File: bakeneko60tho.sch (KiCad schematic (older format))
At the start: 14 parts

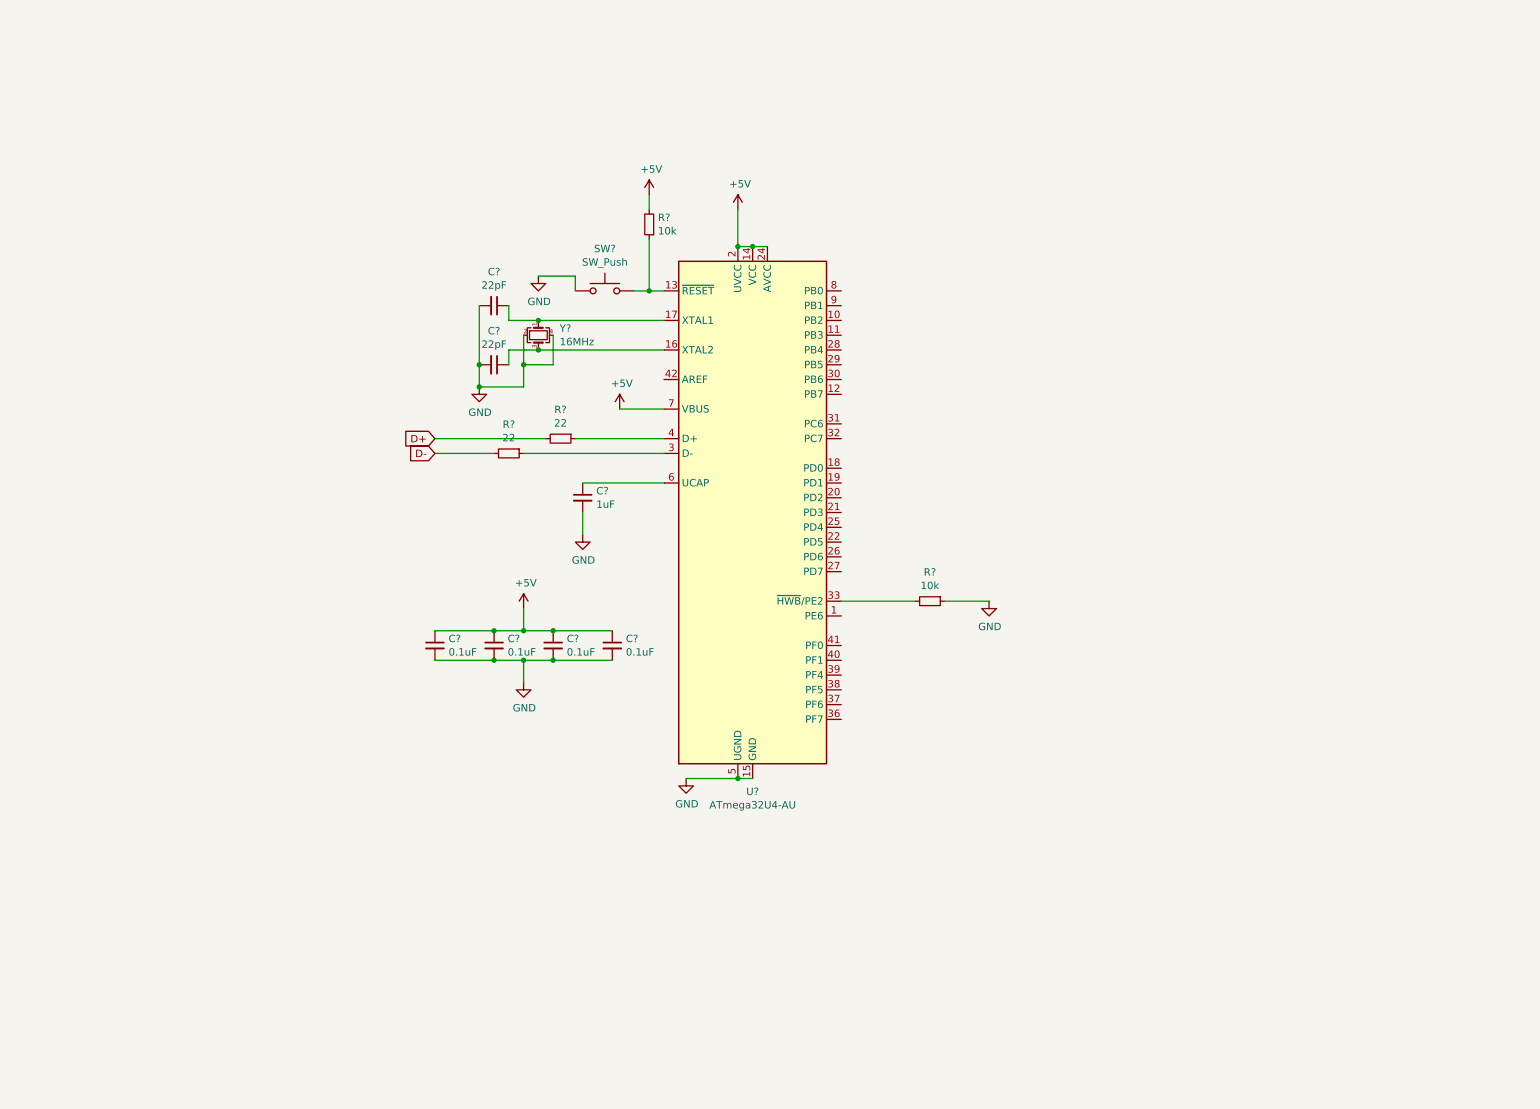
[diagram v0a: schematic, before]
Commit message: assign footprints
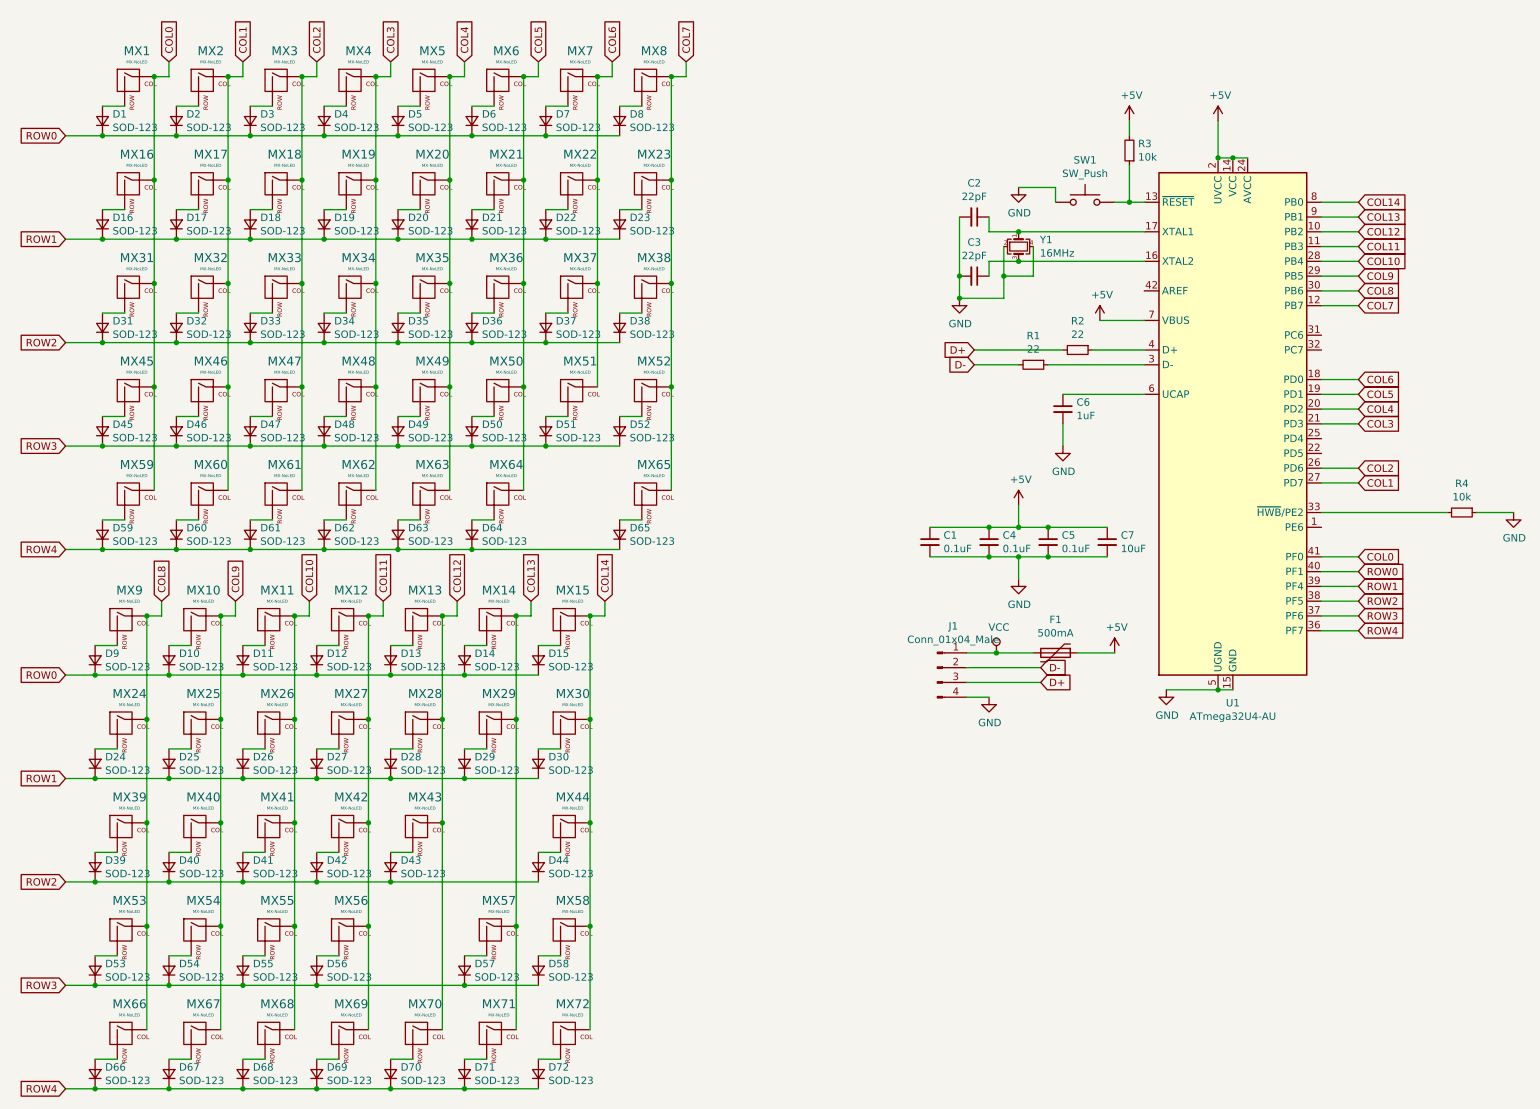
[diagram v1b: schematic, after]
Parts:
- added D1, D10, D11, D12, D13, D14, D15, D16, D17, D18, D19, D2, D20, D21, D22, D23, D24, D25, D26, D27, D28, D29, D3, D30, D31, D32, D33, D34, D35, D36, D37, D38, D39, D4, D40, D41, D42, D43, D44, D45, D46, D47, D48, D49, D5, D50, D51, D52, D53, D54, D55, D56, D57, D58, D59, D6, D60, D61, D62, D63, D64, D65, D66, D67, D68, D69, D7, D70, D71, D72, D8, D9: SOD-123, Diode_SMD:D_SOD-123, symbol Device:D_Small
- added F1: 500mA, Fuse:Fuse_1206_3216Metric, symbol Device:Polyfuse
- added J1: Conn_01x04_Male, Connector_PinHeader_1.00mm:PinHeader_1x04_P1.00mm_Horizontal, symbol Connector:Conn_01x04_Male
- added MX1, MX10, MX11, MX12, MX13, MX14, MX15, MX16, MX17, MX18, MX19, MX2, MX20, MX21, MX22, MX23, MX24, MX25, MX26, MX27, MX28, MX29, MX3, MX30, MX31, MX32, MX33, MX34, MX35, MX36, MX37, MX38, MX39, MX4, MX40, MX41, MX42, MX44, MX45, MX46, MX47, MX48, MX49, MX5, MX50, MX51, MX52, MX53, MX54, MX55, MX57, MX58, MX59, MX6, MX60, MX61, MX62, MX63, MX65, MX66, MX67, MX68, MX69, MX7, MX70, MX71, MX72, MX8, MX9: MX-NoLED, MX_Only:MXOnly-1U-NoLED, symbol MX_Alps_Hybrid:MX-NoLED
- added MX43, MX56: MX-NoLED, MX_Only:MXOnly-2U-NoLED, symbol MX_Alps_Hybrid:MX-NoLED
- added MX64: MX-NoLED, MX_Only:MXOnly-2U-ReversedStabilizers-NoLED, symbol MX_Alps_Hybrid:MX-NoLED
- C1, C2, C3, C4, C5, C6: renamed from C?; footprint (none) -> Capacitor_SMD:C_0805_2012Metric
- C7: renamed from C?; value 0.1uF -> 10uF; footprint (none) -> Capacitor_SMD:C_0805_2012Metric
- R1, R2, R3, R4: renamed from R?; footprint (none) -> Resistor_SMD:R_0805_2012Metric
- Y1: renamed from Y?; footprint (none) -> Crystal:Crystal_SMD_3225-4Pin_3.2x2.5mm
- gave numbers to parts that had none: 2
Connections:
- net +5V: now also F1.1
- net D+: now also J1.3 (Pin_3)
- net D-: now also J1.2 (Pin_2)
- net GND: now also J1.4 (Pin_4)
- net COL12: now reaches U1.10 (PB2)
- net COL12: now also MX13.1 (COL), MX28.1 (COL), MX43.1 (COL), MX70.1 (COL)
- net COL11: now reaches U1.11 (PB3)
- net COL11: now also MX12.1 (COL), MX27.1 (COL), MX42.1 (COL), MX56.1 (COL), MX69.1 (COL)
- net COL7: now reaches U1.12 (PB7)
- net COL7: now also MX23.1 (COL), MX38.1 (COL), MX52.1 (COL), MX65.1 (COL), MX8.1 (COL)
- net COL6: now reaches U1.18 (PD0)
- net COL6: now also MX22.1 (COL), MX37.1 (COL), MX51.1 (COL), MX7.1 (COL)
- net COL5: now reaches U1.19 (PD1)
- net COL5: now also MX21.1 (COL), MX36.1 (COL), MX50.1 (COL), MX6.1 (COL), MX64.1 (COL)
- net COL4: now reaches U1.20 (PD2)
- net COL4: now also MX20.1 (COL), MX35.1 (COL), MX49.1 (COL), MX5.1 (COL), MX63.1 (COL)
- net COL3: now reaches U1.21 (PD3)
- net COL3: now also MX19.1 (COL), MX34.1 (COL), MX4.1 (COL), MX48.1 (COL), MX62.1 (COL)
- net COL2: now reaches U1.26 (PD6)
- net COL2: now also MX18.1 (COL), MX3.1 (COL), MX33.1 (COL), MX47.1 (COL), MX61.1 (COL)
- net COL1: now reaches U1.27 (PD7)
- net COL1: now also MX17.1 (COL), MX2.1 (COL), MX32.1 (COL), MX46.1 (COL), MX60.1 (COL)
- net COL10: now reaches U1.28 (PB4)
- net COL10: now also MX11.1 (COL), MX26.1 (COL), MX41.1 (COL), MX55.1 (COL), MX68.1 (COL)
- net COL9: now reaches U1.29 (PB5)
- net COL9: now also MX10.1 (COL), MX25.1 (COL), MX40.1 (COL), MX54.1 (COL), MX67.1 (COL)
- net COL8: now reaches U1.30 (PB6)
- net COL8: now also MX24.1 (COL), MX39.1 (COL), MX53.1 (COL), MX66.1 (COL), MX9.1 (COL)
- net ROW4: now reaches U1.36 (PF7)
- net ROW4: now also D59.1 (K), D60.1 (K), D61.1 (K), D62.1 (K), D63.1 (K), D64.1 (K), D65.1 (K), D66.1 (K), D67.1 (K), D68.1 (K), D69.1 (K), D70.1 (K), D71.1 (K), D72.1 (K)
- net ROW3: now reaches U1.37 (PF6)
- net ROW3: now also D45.1 (K), D46.1 (K), D47.1 (K), D48.1 (K), D49.1 (K), D50.1 (K), D51.1 (K), D52.1 (K), D53.1 (K), D54.1 (K), D55.1 (K), D56.1 (K), D57.1 (K), D58.1 (K)
- net ROW2: now reaches U1.38 (PF5)
- net ROW2: now also D31.1 (K), D32.1 (K), D33.1 (K), D34.1 (K), D35.1 (K), D36.1 (K), D37.1 (K), D38.1 (K), D39.1 (K), D40.1 (K), D41.1 (K), D42.1 (K), D43.1 (K), D44.1 (K)
- net ROW1: now reaches U1.39 (PF4)
- net ROW1: now also D16.1 (K), D17.1 (K), D18.1 (K), D19.1 (K), D20.1 (K), D21.1 (K), D22.1 (K), D23.1 (K), D24.1 (K), D25.1 (K), D26.1 (K), D27.1 (K), D28.1 (K), D29.1 (K), D30.1 (K)
- net ROW0: now reaches U1.40 (PF1)
- net ROW0: now also D1.1 (K), D10.1 (K), D11.1 (K), D12.1 (K), D13.1 (K), D14.1 (K), D15.1 (K), D2.1 (K), D3.1 (K), D4.1 (K), D5.1 (K), D6.1 (K), D7.1 (K), D8.1 (K), D9.1 (K)
- net COL0: now reaches U1.41 (PF0)
- net COL0: now also MX1.1 (COL), MX16.1 (COL), MX31.1 (COL), MX45.1 (COL), MX59.1 (COL)
- net COL14: now reaches U1.8 (PB0)
- net COL14: now also MX15.1 (COL), MX30.1 (COL), MX44.1 (COL), MX58.1 (COL), MX72.1 (COL)
- net COL13: now reaches U1.9 (PB1)
- net COL13: now also MX14.1 (COL), MX29.1 (COL), MX57.1 (COL), MX71.1 (COL)
- new net: D36.2 (A), MX36.2 (ROW)
- new net: D37.2 (A), MX37.2 (ROW)
- new net: D38.2 (A), MX38.2 (ROW)
- new net: D39.2 (A), MX39.2 (ROW)
- new net: D40.2 (A), MX40.2 (ROW)
- new net: D41.2 (A), MX41.2 (ROW)
- new net: D42.2 (A), MX42.2 (ROW)
- new net: D43.2 (A), MX43.2 (ROW)
- new net: D44.2 (A), MX44.2 (ROW)
- new net: D31.2 (A), MX31.2 (ROW)
- new net: D32.2 (A), MX32.2 (ROW)
- new net: D33.2 (A), MX33.2 (ROW)
- new net: D34.2 (A), MX34.2 (ROW)
- new net: D35.2 (A), MX35.2 (ROW)
- new net: D50.2 (A), MX50.2 (ROW)
- new net: D51.2 (A), MX51.2 (ROW)
- new net: D52.2 (A), MX52.2 (ROW)
- new net: D53.2 (A), MX53.2 (ROW)
- new net: D54.2 (A), MX54.2 (ROW)
- new net: D55.2 (A), MX55.2 (ROW)
- new net: D56.2 (A), MX56.2 (ROW)
- new net: D57.2 (A), MX57.2 (ROW)
- new net: D58.2 (A), MX58.2 (ROW)
- new net: D45.2 (A), MX45.2 (ROW)
- new net: D46.2 (A), MX46.2 (ROW)
- new net: D47.2 (A), MX47.2 (ROW)
- new net: D48.2 (A), MX48.2 (ROW)
- new net: D49.2 (A), MX49.2 (ROW)
- new net: D64.2 (A), MX64.2 (ROW)
- new net: D65.2 (A), MX65.2 (ROW)
- new net: D66.2 (A), MX66.2 (ROW)
- new net: D67.2 (A), MX67.2 (ROW)
- new net: D68.2 (A), MX68.2 (ROW)
- new net: D69.2 (A), MX69.2 (ROW)
- new net: D70.2 (A), MX70.2 (ROW)
- new net: D71.2 (A), MX71.2 (ROW)
- new net: D72.2 (A), MX72.2 (ROW)
- new net: D59.2 (A), MX59.2 (ROW)
- new net: D60.2 (A), MX60.2 (ROW)
- new net: D61.2 (A), MX61.2 (ROW)
- new net: D62.2 (A), MX62.2 (ROW)
- new net: D63.2 (A), MX63.2 (ROW)
- new net: D6.2 (A), MX6.2 (ROW)
- new net: D7.2 (A), MX7.2 (ROW)
- new net: D8.2 (A), MX8.2 (ROW)
- new net: D9.2 (A), MX9.2 (ROW)
- new net: D10.2 (A), MX10.2 (ROW)
- new net: D11.2 (A), MX11.2 (ROW)
- new net: D12.2 (A), MX12.2 (ROW)
- new net: D13.2 (A), MX13.2 (ROW)
- new net: D14.2 (A), MX14.2 (ROW)
- new net: D15.2 (A), MX15.2 (ROW)
- new net: D1.2 (A), MX1.2 (ROW)
- new net: D2.2 (A), MX2.2 (ROW)
- new net: D3.2 (A), MX3.2 (ROW)
- new net: D4.2 (A), MX4.2 (ROW)
- new net: D5.2 (A), MX5.2 (ROW)
- new net: D21.2 (A), MX21.2 (ROW)
- new net: D22.2 (A), MX22.2 (ROW)
- new net: D23.2 (A), MX23.2 (ROW)
- new net: D24.2 (A), MX24.2 (ROW)
- new net: D25.2 (A), MX25.2 (ROW)
- new net: D26.2 (A), MX26.2 (ROW)
- new net: D27.2 (A), MX27.2 (ROW)
- new net: D28.2 (A), MX28.2 (ROW)
- new net: D29.2 (A), MX29.2 (ROW)
- new net: D30.2 (A), MX30.2 (ROW)
- new net: D16.2 (A), MX16.2 (ROW)
- new net: D17.2 (A), MX17.2 (ROW)
- new net: D18.2 (A), MX18.2 (ROW)
- new net: D19.2 (A), MX19.2 (ROW)
- new net: D20.2 (A), MX20.2 (ROW)
- new net VCC: F1.2, J1.1 (Pin_1)
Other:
- moved on the sheet: C1, C2, C3, C4, C5, C6, C7, R1, R2, R3, R4, SW1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
